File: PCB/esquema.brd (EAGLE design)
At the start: 97.8 x 86 mm, 11 parts, among them U1 ATMEGA328P_TQFP

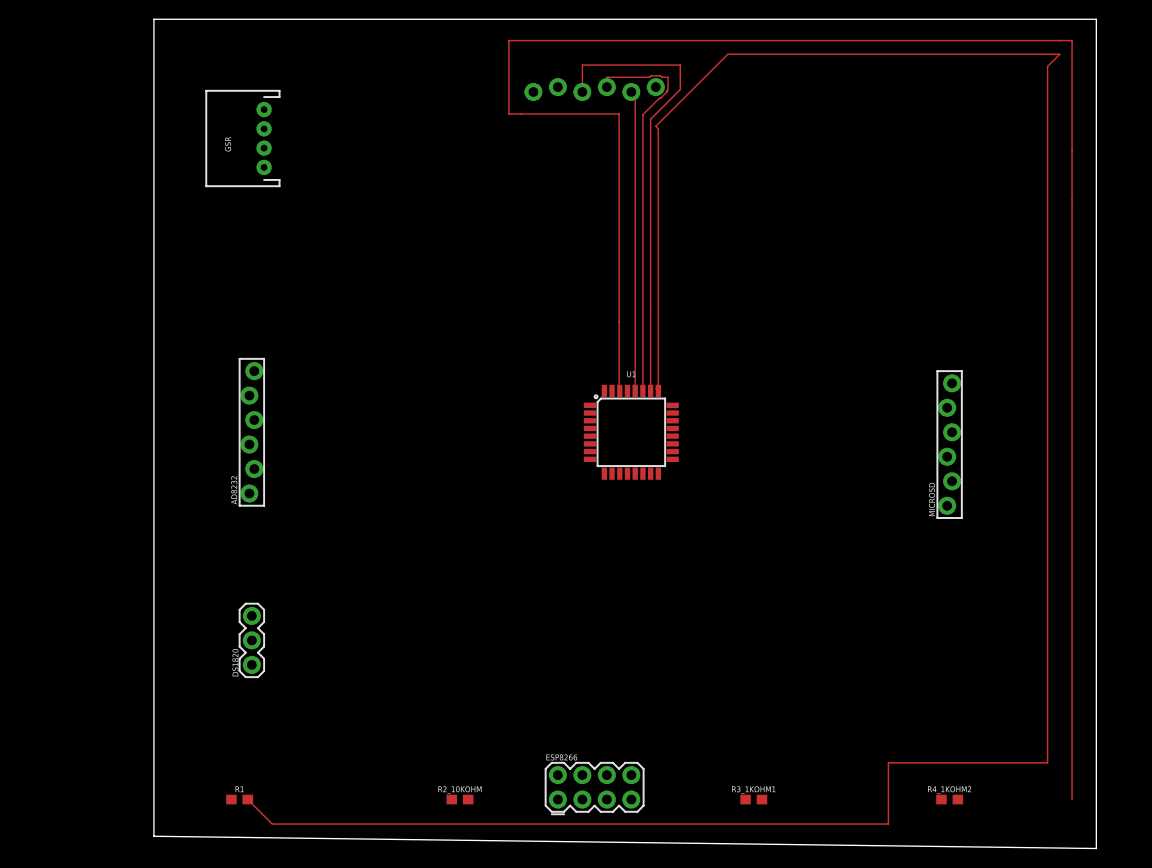
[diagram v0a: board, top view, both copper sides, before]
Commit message: Fin PCB
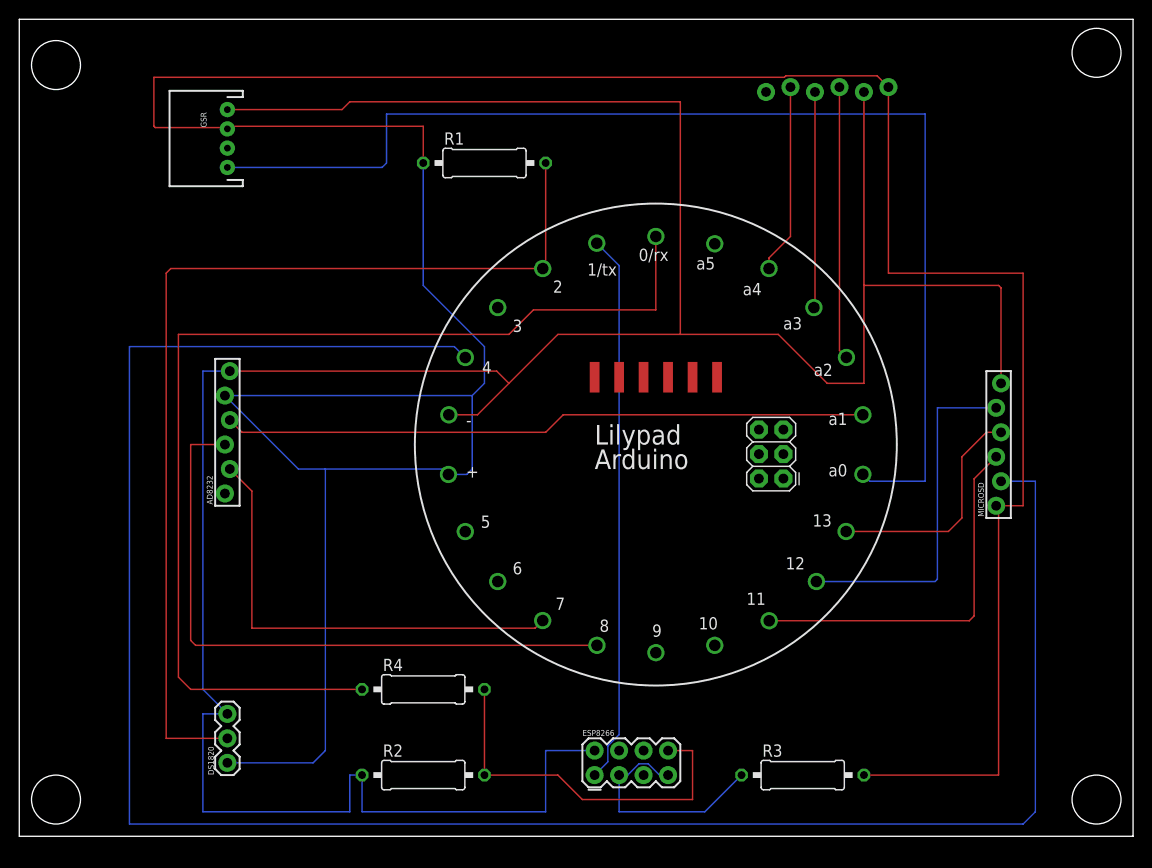
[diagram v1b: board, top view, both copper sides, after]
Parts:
- removed R2_10KOHM, R3_1KOHM1, R4_1KOHM2: 2.2MOHM-1/10W-5%(0603), SparkFun-Retired:0603
- removed U1: ATMEGA328P_TQFP, SparkFun-IC-Microcontroller:TQFP32-08
- added PCB1: ARDUINO_LILYPAD, E14_Arduino_revB:ARDUINO_LILYPAD
- added R2, R4: 1K, rcl:0309/12
- added R3: 10K, rcl:0309/12
- R1: value 4.7OHM-1/10W-5%(0603) -> 4.7K; device SparkFun-Retired:0603 -> rcl:0309/12
- moved R1 70.8 mm to (55.9, 68.6)
- moved ADXL335 36.8 mm to (97.8, 76.2), turned to 0 degrees
- moved DS1820 10.5 mm to (29.2, 6.35)
- moved MICROSD 5.08 mm to (109.2, 33.0)
- moved ESP8266 4.58 mm to (71.1, 6.35)
- moved GSR 3.81 mm to (29.2, 71.1)
- moved AD8232 2.54 mm to (29.2, 34.3)
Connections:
- removed net 3.3V: AD8232.5, ADXL335.1, DS1820.1, GSR.3, MICROSD.1, R1.1, R2_10KOHM.2, U1.4, U1.6
- new net N$18: MICROSD.5, PCB1.12
- net N$1: now also MICROSD.3, PCB1.11; no longer AD8232.6, ADXL335.2, DS1820.3, ESP8266.2, GSR.4, MICROSD.6, R3_1KOHM1.1, U1.3, U1.5
- net N$10: now also R3.1; no longer R2_10KOHM.1
- net N$11: now also ADXL335.5, PCB1.A4; no longer ESP8266.1, U1.31
- net N$12: now also ESP8266.1, PCB1.1/TX; no longer ESP8266.8, R3_1KOHM1.2, R4_1KOHM2.1
- net N$13: now also ESP8266.8, R2.2, R4.2; no longer AD8232.2, U1.11
- net N$14: now also PCB1.0/RX, R4.1; no longer R4_1KOHM2.2, U1.30
- net N$15: now also AD8232.5, ADXL335.1, DS1820.1, GSR.3, MICROSD.1, PCB1.+, R1.1, R3.2; no longer MICROSD.2, U1.16
- net N$16: now also AD8232.6, ADXL335.2, DS1820.3, ESP8266.2, GSR.4, MICROSD.6, PCB1.-, R2.1; no longer MICROSD.3, U1.17
- net N$17: now also PCB1.13; no longer U1.15
- net N$2: now also MICROSD.2, PCB1.4; no longer GSR.1, U1.23
- net N$3: now also GSR.1, PCB1.A0; no longer AD8232.4, U1.24
- net N$4: now also AD8232.4, PCB1.A1; no longer AD8232.3, U1.12
- net N$5: now also AD8232.3, PCB1.8; no longer MICROSD.5, U1.2
- net N$6: now also AD8232.2, PCB1.7; no longer ADXL335.3, U1.26
- net N$7: now also PCB1.2; no longer U1.25
- net N$8: now also ADXL335.3, PCB1.A2; no longer ADXL335.4, U1.27
- net N$9: now also ADXL335.4, PCB1.A3; no longer ADXL335.5, U1.28
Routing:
- net N$15: track 0.00 -> 345.5 mm
- net N$16: track 0.00 -> 310.7 mm
- net N$2: track 0.00 -> 217.2 mm
- net N$7: track 237.3 -> 105.0 mm
- net N$3: track 0.41 -> 122.5 mm
- net N$14: track 185.1 -> 113.3 mm
- net N$4: track 0.00 -> 67.0 mm
- net N$5: track 0.00 -> 66.2 mm
- net N$12: track 0.00 -> 57.2 mm
- net N$13: track 0.00 -> 39.2 mm
- net N$1: track 0.00 -> 38.9 mm
- net N$18: track 0.00 -> 36.5 mm
- net N$10: track 0.00 -> 24.1 mm
- net N$17: track 0.00 -> 24.1 mm
- net N$11: track 0.00 -> 19.7 mm
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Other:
- board size 97.8 x 86 mm -> 115.5 x 84.8 mm
